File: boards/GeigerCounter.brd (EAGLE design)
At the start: 71.8 x 55.2 mm, 40 parts, among them IC1 TLC555CP, IC2 ATtiny2313A-SU, J1 I2C, J2 ICSP, J3 I/O, Q1 LND 712, Q2 STN83003, Q3 MMBT2222ALT3G, Q4 MMBT2222ALT3G, Q5 8 MHz, Q6 SMD Buzzer

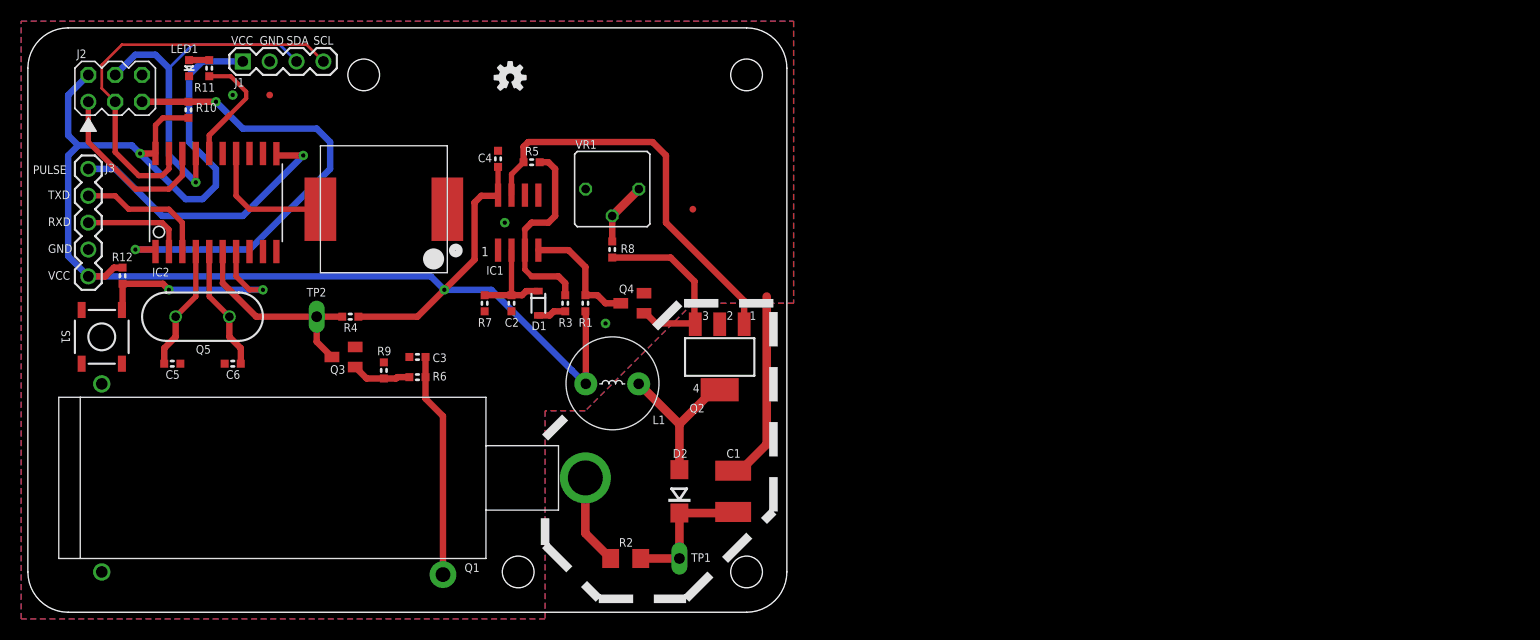
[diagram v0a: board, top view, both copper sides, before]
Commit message: put all the downloaded files into directories
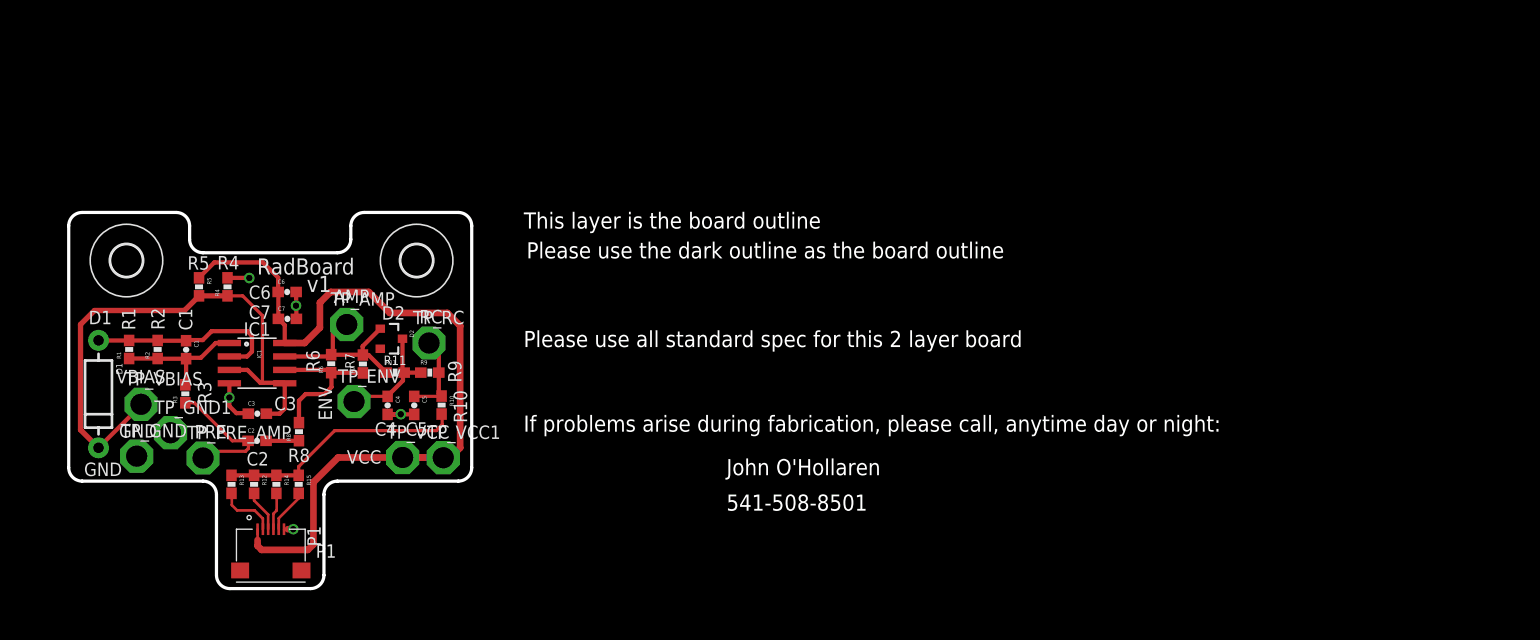
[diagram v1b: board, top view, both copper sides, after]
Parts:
- removed IC2: ATtiny2313A-SU, avr-6:SO20L$
- removed J1: I2C, freetronics-master-v1:1X04
- removed J2: ICSP, connectors:ICSP-6
- removed J3: I/O, freetronics-master-v1:1X05
- removed JP1, JP2: FIDUCIALUFIDUCIAL, SparkFun:MICRO-FIDUCIAL
- removed L1: 10mH, Luke:INDUCTOR-5.08
- removed LED1: Event, freetronics-master-v1:LED-0603
- removed Q1: LND 712, SparkFun:GEIGER_TUBE
- removed Q2: STN83003, transistor-neu-to92:SOT223
- removed Q3, Q4: MMBT2222ALT3G, SparkFun:SOT23
- removed Q5: 8 MHz, freetronics-master-v1:HC49US
- removed Q6: SMD Buzzer, freetronics-master-v1:BUZZER-12X12-SMT
- removed S1: Mute, SparkFun:TACTILE_SWITCH_SMD
- removed SY: OSHW-LOGOS, SparkFun:OSHW-LOGO-S
- removed TP1: HV, connectors:TP_PTH
- removed TP2: GM Pulse, connectors:TP_PTH
- removed VR1: 10Ω, pot:CT6
- added C7: 0.1uF, SparkFun-Passives:0603-CAP
- added H1, H2: MOUNT-HOLE3.0, holes:3,0
- added P1: XF2M-0615-1A, GeigerCounter:XF2M-0615-1A
- added R13, R14, R15: 0, SparkFun-Passives:0603-RES
- added TP_AMP, TP_ENV, TP_GND, TP_GND1, TP_PRE_AMP, TP_RC, TP_VBIAS, TP_VCC, TP_VCC1: PTR1PAD1-20, testpad:P1-20
- C1: value 10nF -> 15pF; device rcl:C1812 -> SparkFun-Passives:0603-CAP
- C2: value 1nF -> 100p; device freetronics-master-v1:0603 -> SparkFun-Passives:0603-CAP
- C3: value 220pF -> 0.1u; device freetronics-master-v1:0603 -> SparkFun-Passives:0603-CAP
- C4: value 100nF -> DNP; device freetronics-master-v1:0603 -> SparkFun-Passives:0603-CAP
- C5: value 22pF -> DNP; device freetronics-master-v1:0603 -> SparkFun-Passives:0603-CAP
- C6: value 22pF -> 2.2uF; device freetronics-master-v1:0603 -> SparkFun-Passives:0603-CAP
- D1: value 1N4148WS -> S1223; device SparkFun:SOD-323 -> GeigerCounter:DIODE-1N4001
- D2: value RS1M -> DNP; device diode:DO214AC -> SparkFun-DiscreteSemi:SOT23-3
- IC1: value TLC555CP -> OPAMP-DUALU; device linear:SO08 -> SparkFun-AnalogIC:SO08
- R1: value 100kΩ -> 10M; device freetronics-master-v1:0603 -> SparkFun-Passives:0603-RES
- R10, R12: value 10kΩ -> 0; device freetronics-master-v1:0603 -> SparkFun-Passives:0603-RES
- R11: value 100Ω -> 0; device freetronics-master-v1:0603 -> SparkFun-Passives:0603-RES
- R2: value 4.7MΩ -> DNP; device rcl:R1206 -> SparkFun-Passives:0603-RES
- R3: value 1kΩ -> 0; device freetronics-master-v1:0603 -> SparkFun-Passives:0603-RES
- R4: value 10kΩ -> 100; device freetronics-master-v1:0603 -> SparkFun-Passives:0603-RES
- R5: value 330Ω -> 100; device freetronics-master-v1:0603 -> SparkFun-Passives:0603-RES
- R6: value 22kΩ -> 100k; device freetronics-master-v1:0603 -> SparkFun-Passives:0603-RES
- R7: value 220kΩ -> DNP; device freetronics-master-v1:0603 -> SparkFun-Passives:0603-RES
- R8: value 15Ω -> 10k; device freetronics-master-v1:0603 -> SparkFun-Passives:0603-RES
- R9: value 100k -> 0; device freetronics-master-v1:0603 -> SparkFun-Passives:0603-RES
- moved C1 53.4 mm to (14.3, 26.1), turned to 270 degrees
- moved R2 48.5 mm to (11.6, 26.1), turned to 90 degrees
- moved R1 43.3 mm to (8.94, 26.1)
- moved D1 42.5 mm to (6.05, 21.9)
- moved R3 36.9 mm to (14.2, 21.9)
- moved R10 36.8 mm to (38.5, 20.9)
- moved R8 34.3 mm to (25.0, 18.3), turned to 90 degrees
- moved R11 33.7 mm to (34.1, 23.9), turned to 0 degrees
- moved R5 33.6 mm to (15.5, 32.0), turned to 270 degrees
- moved D2 30.9 mm to (33.7, 27.1), turned to 270 degrees
- moved IC1 28.0 mm to (21.0, 24.8), turned to 270 degrees
- moved C2 27.3 mm to (21.0, 17.5), turned to 0 degrees
- moved C4 25.5 mm to (33.4, 20.8), turned to 270 degrees
- moved R12 23.3 mm to (20.8, 13.4)
- moved C5 23.2 mm to (35.9, 20.8), turned to 270 degrees
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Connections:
- removed net !RESET: IC2.1, J2.5, R10.1
- removed net +3V3: C4.1, IC1.8, IC2.20, J1.1, J2.2, J3.1, L1.1, R1.1, R10.2, R12.1, R4.2
- removed net GM_PULSE: IC2.6, Q3.3, R4.1, TP2.P$1
- removed net MUTE1: IC2.7, R12.2, S1.1
- removed net N$1: Q1.VCC, R2.1
- removed net N$14: IC1.7, Q2.1, R5.2
- removed net N$15: IC1.4, Q4.3, R1.2
- removed net N$26: IC2.2, J3.3
- removed net N$27: IC2.3, J3.4
- removed net N$28: C6.1, IC2.5, Q5.1
- removed net N$29: C5.1, IC2.4, Q5.2
- removed net N$31: IC2.18, J2.1
- removed net N$33: IC2.16, R11.2
- removed net N$34: LED1.A, R11.1
- removed net N$35: IC2.14, Q6.2
- removed net N$39: IC1.3, R3.2, R5.1
- removed net N$48: C3.1, Q1.GND, R6.2
- removed net N$49: Q3.1, R6.1, R9.2
- removed net N$50: C2.1, D1.1, IC1.2, R7.2
- removed net N$54: D1.2, R3.1
- removed net N$55: Q2.3, Q4.1, R8.2
- removed net N$56: R8.1, VR1.A, VR1.S
- removed net N$57: D2.A, L1.2, Q2.4
- removed net N$58: C1.1, D2.C, R2.2, TP1.P$1
- removed net PULSE: IC2.11, J3.5
- removed net SCL: IC2.19, J1.4, J2.3
- removed net SDA: IC2.17, J1.3, J2.4
- new net ENV_DETEC_OUT: C4.1, D2.3, R11.2, R9.1, TP_ENV.TP
- new net IC1A_N: C1.1, D1.A, IC1.2, R1.2, R2.2
- new net IC1A_OUT: C1.2, IC1.1, R1.1, R2.1, R3.2
- new net IC1B_N: IC1.6, R6.1, R7.1, R8.2
- new net IC1B_OUT: D2.1, IC1.7, R11.1, R6.2, R7.2, TP_AMP.TP
- new net INV_AMP_INPUT: C2.2, R8.1
- new net NC1: P1.2, R13.2
- new net NC2: P1.4, R14.2
- new net OUTPUT: R10.2, R12.1, R13.1, R14.1, R15.1
- new net P3.4: P1.5, R15.2
- new net P3.5: P1.3, R12.2
- new net PRE_AMP: C2.1, R3.1, TP_PRE_AMP.TP
- new net RC_OUT: C5.1, R10.1, R9.2, TP_RC.TP
- new net VCC: C6.1, C7.1, IC1.8, P1.1, R5.1, TP_VCC.TP, TP_VCC1.TP
- new net VCC_1.25: C3.2, D1.C, IC1.3, IC1.5, R4.1, R5.2, TP_VBIAS.TP
- net GND: now also C3.1, C7.2, IC1.4, P1.6, R4.2, TP_GND.TP, TP_GND1.TP; no longer C1.2, C2.2, C3.2, IC1.1, IC1.6, IC2.10, J1.2, J2.6, J3.2, LED1.C, Q3.2, Q4.2, Q6.1, R7.1, R9.1, S1.3, VR1.E
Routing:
- net +3V3: track 147.3 -> 0.00 mm, vias 2 -> 0
- net VCC: track 0.00 -> 80.1 mm
- net VCC_1.25: track 0.00 -> 53.7 mm
- net !RESET: track 45.5 -> 0.00 mm, vias 2 -> 0
- net SCL: track 38.9 -> 0.00 mm
- net N$14: track 38.2 -> 0.00 mm
- net SDA: track 34.6 -> 0.00 mm, vias 1 -> 0
- net PULSE: track 27.1 -> 0.00 mm, vias 1 -> 0
- net OUTPUT: track 0.00 -> 23.4 mm
- net MUTE1: track 21.4 -> 0.00 mm, vias 2 -> 0
- net N$48: track 21.3 -> 0.00 mm
- net GM_PULSE: track 20.0 -> 0.00 mm
- net IC1A_N: track 0.00 -> 19.0 mm
- net N$39: track 18.8 -> 0.00 mm
- net N$55: track 17.9 -> 0.00 mm
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- removed copper zone on layer 1, net GND
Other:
- board size 71.8 x 55.2 mm -> 38.1 x 35.6 mm
- board text added: "541-508-8501"
- board text added: "AMP"
- board text added: "C1"
- board text added: "C2"
- board text added: "C3"
- board text added: "C4"
- board text added: "C5"
- board text added: "C6"
- board text added: "C7"
- board text added: "D1"
- board text added: "D2"
- board text added: "ENV"
- board text added: "IC1"
- board text added: "If problems arise during fabrication, please call, anytime day or night:"
- board text added: "John O'Hollaren"
- board text added: "P1"
- board text added: "PRE"
- board text added: "Please use all standard spec for this 2 layer board"
- board text added: "Please use the dark outline as the board outline"
- board text added: "R1"
- board text added: "R10"
- board text added: "R11"
- board text added: "R2"
- board text added: "R3"
- board text added: "R4"
- board text added: "R5"
- board text added: "R6"
- board text added: "R7"
- board text added: "R8"
- board text added: "R9"
- board text added: "RC"
- board text added: "RadBoard"
- board text added: "This layer is the board outline"
- board text added: "VBIAS"
- board text added: "v1"
- board text removed: "1"
- board text removed: "PULSE"
- board text removed: "RXD"
- board text removed: "SCL"
- board text removed: "SDA"
- board text removed: "TXD"
